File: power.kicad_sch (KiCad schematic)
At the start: 40 parts, among them Q2 SQJQ131EL, Q3 2N7002KT1G, U4 5V 200mA, U5 3.3V 200mA, U6 TLV709A50DBVR

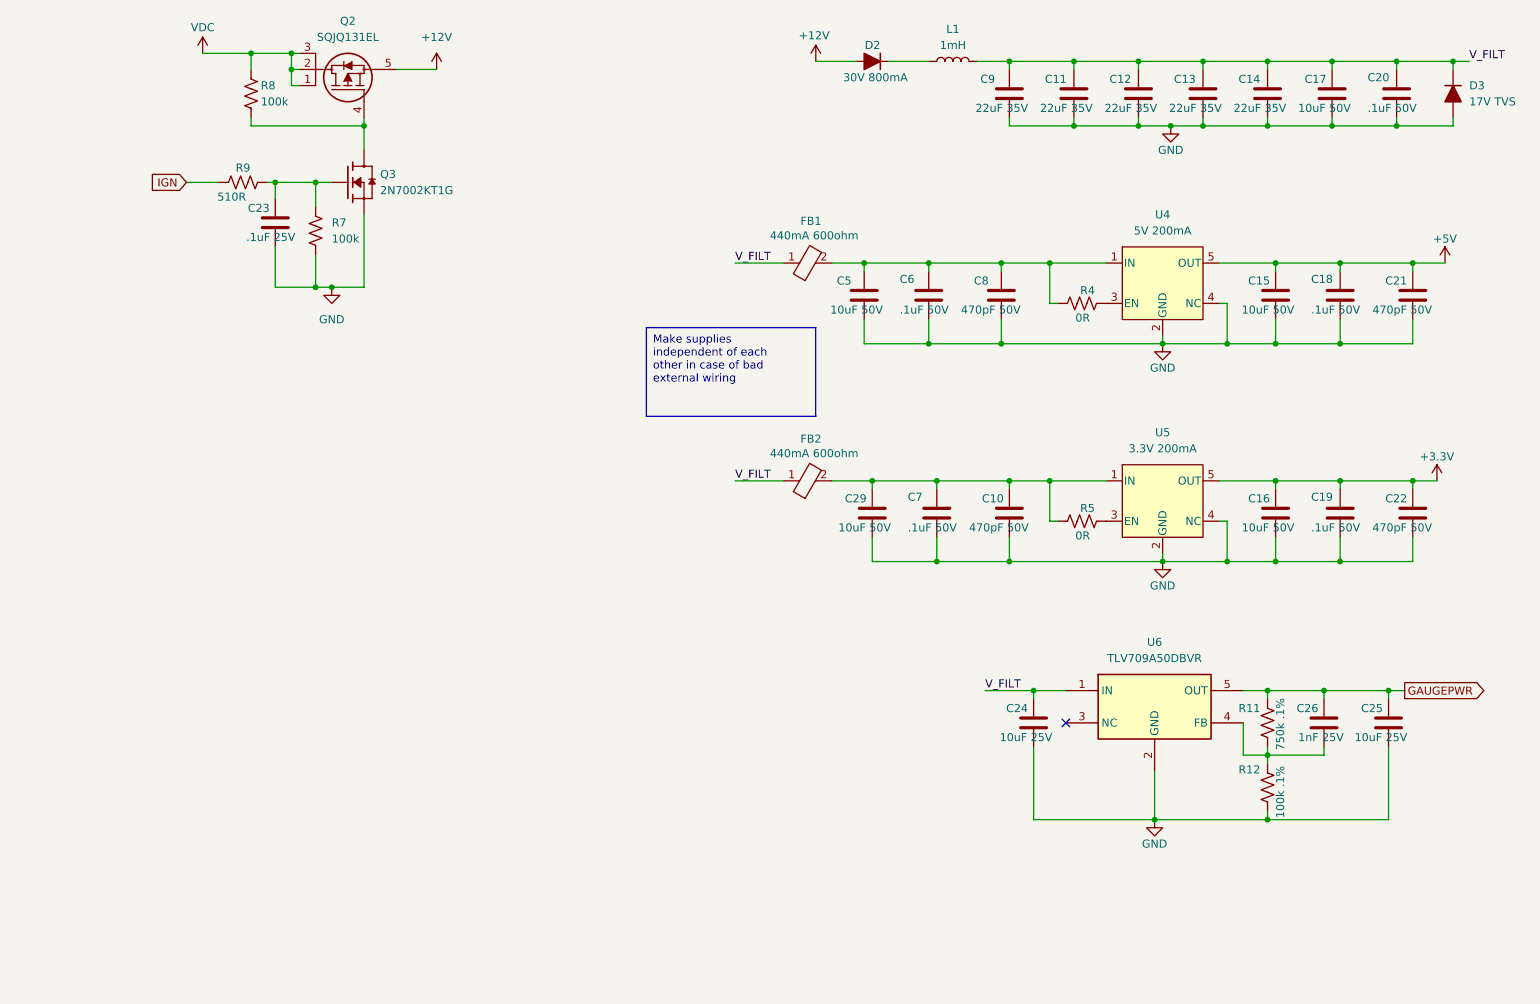
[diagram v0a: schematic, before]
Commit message: Initial schematic is done
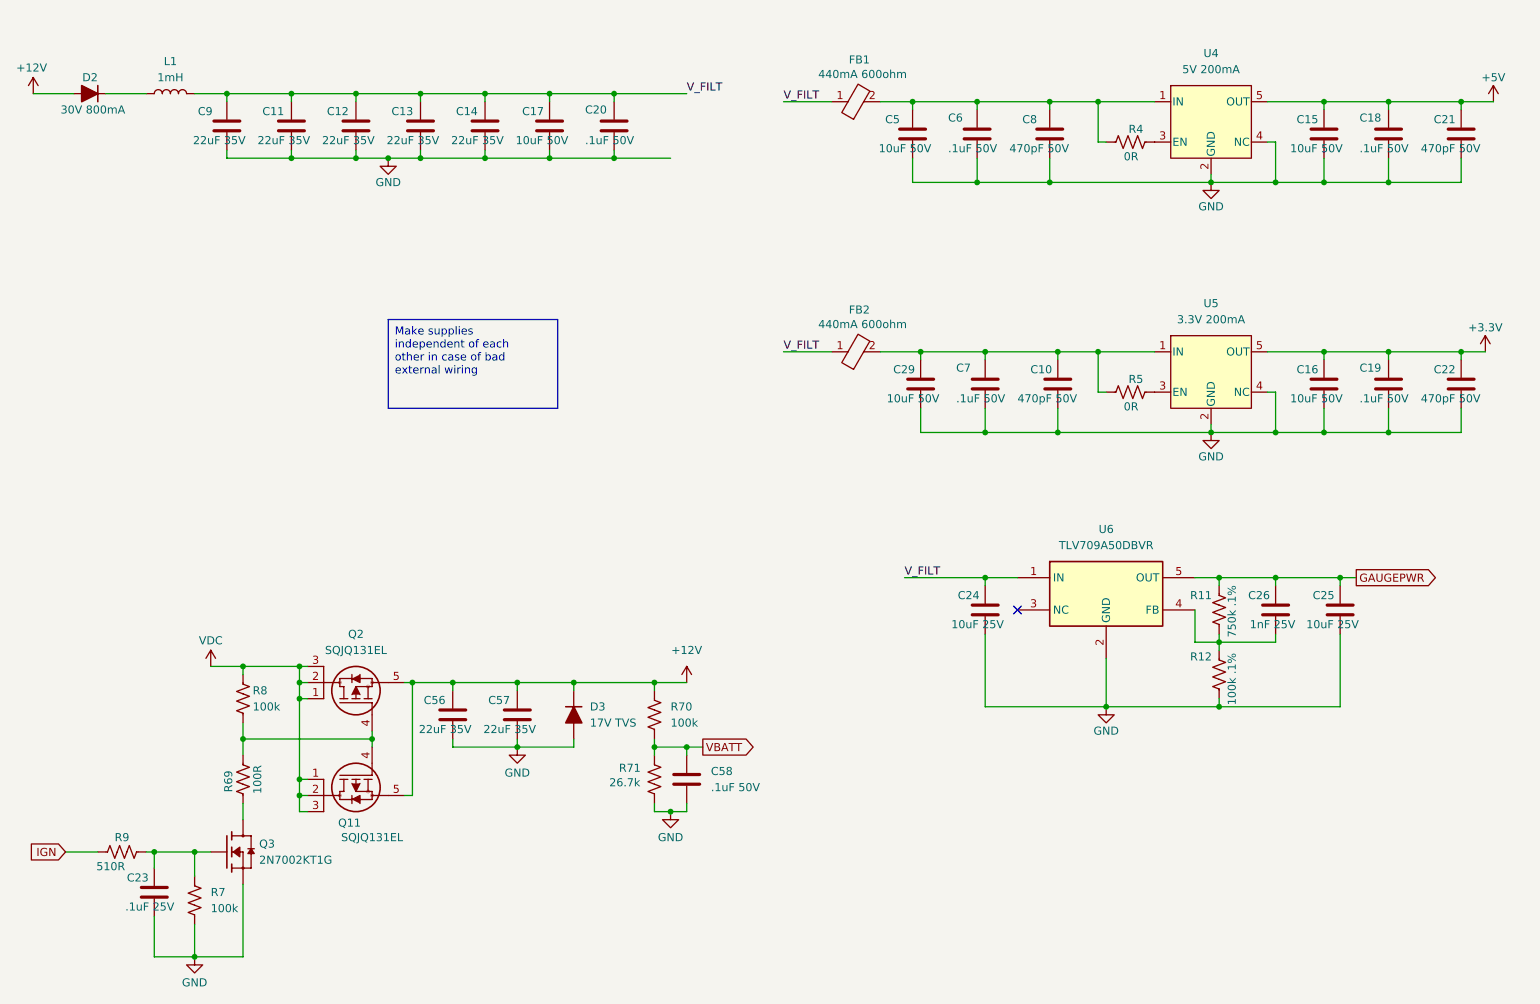
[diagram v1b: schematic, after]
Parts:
- added C56, C57: 22uF 35V, Sullivan-Labs:C_0805_2012Metric, symbol Sullivan-Labs:CAP_22uF_35V_0805
- added C58: .1uF 50V, Sullivan-Labs:C_0402_1005Metric, symbol Sullivan-Labs:CAP_.1uF_50V_0402
- added Q11: SQJQ131EL, Sullivan-Labs:TO_EL-T1_GE3_VIS, symbol Sullivan-Labs:PMOS SQJQ131EL
- added R69: 100R, Sullivan-Labs:R_0402_1005Metric, symbol Sullivan-Labs:RES_100R_0402
- added R70: 100k, Sullivan-Labs:R_0402_1005Metric, symbol Sullivan-Labs:RES_100k_0402
- added R71: 26.7k, Sullivan-Labs:R_0402_1005Metric, symbol Sullivan-Labs:RES_26.7k_0402
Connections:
- net +12V: now also D3.1 (K), C56.1, C57.1, Q11.5, R70.1
- net GND: now also C56.2, C57.2, C58.2, R71.2
- net VDC: now also Q11.1, Q11.2, Q11.3
- net V_FILT: no longer D3.1 (K)
- net at Q2.4, R8.2: now also Q11.4, R69.1; no longer Q3.3 (D)
- new net: Q3.3 (D), R69.2
- new net VBATT: C58.1, R70.2, R71.1
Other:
- moved on the sheet: C10, C11, C12, C13, C14, C15, C16, C17, C18, C19, C20, C21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
